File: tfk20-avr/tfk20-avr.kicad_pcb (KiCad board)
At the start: 4 copper layers, 76.2 x 115.5 mm, 123 parts, among them J1 USB_C_Receptacle_USB2.0, J2 AVR-ISP-6, SW1 Reset, U1 ATmega32U4-AU, U2 IS31FL3733-TQ, Y1 16MHz

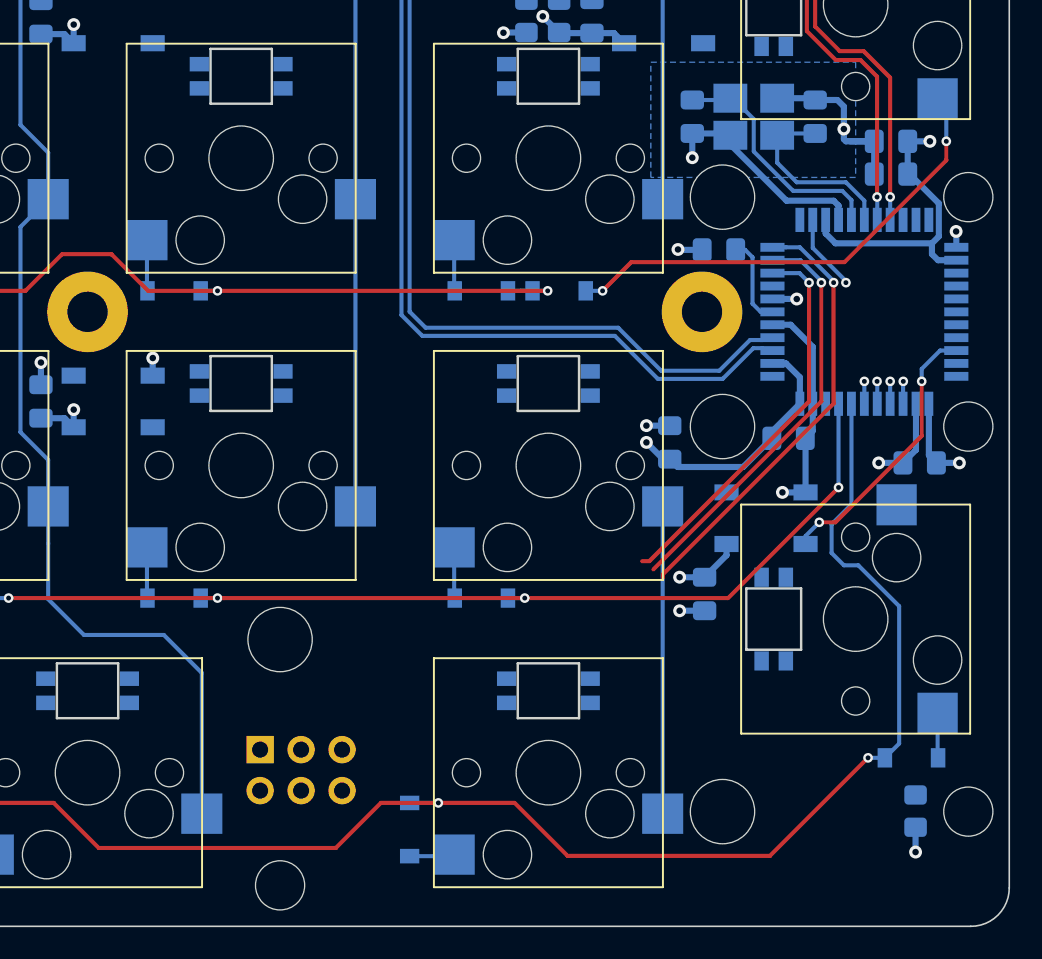
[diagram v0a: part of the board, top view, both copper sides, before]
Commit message: Continue routing
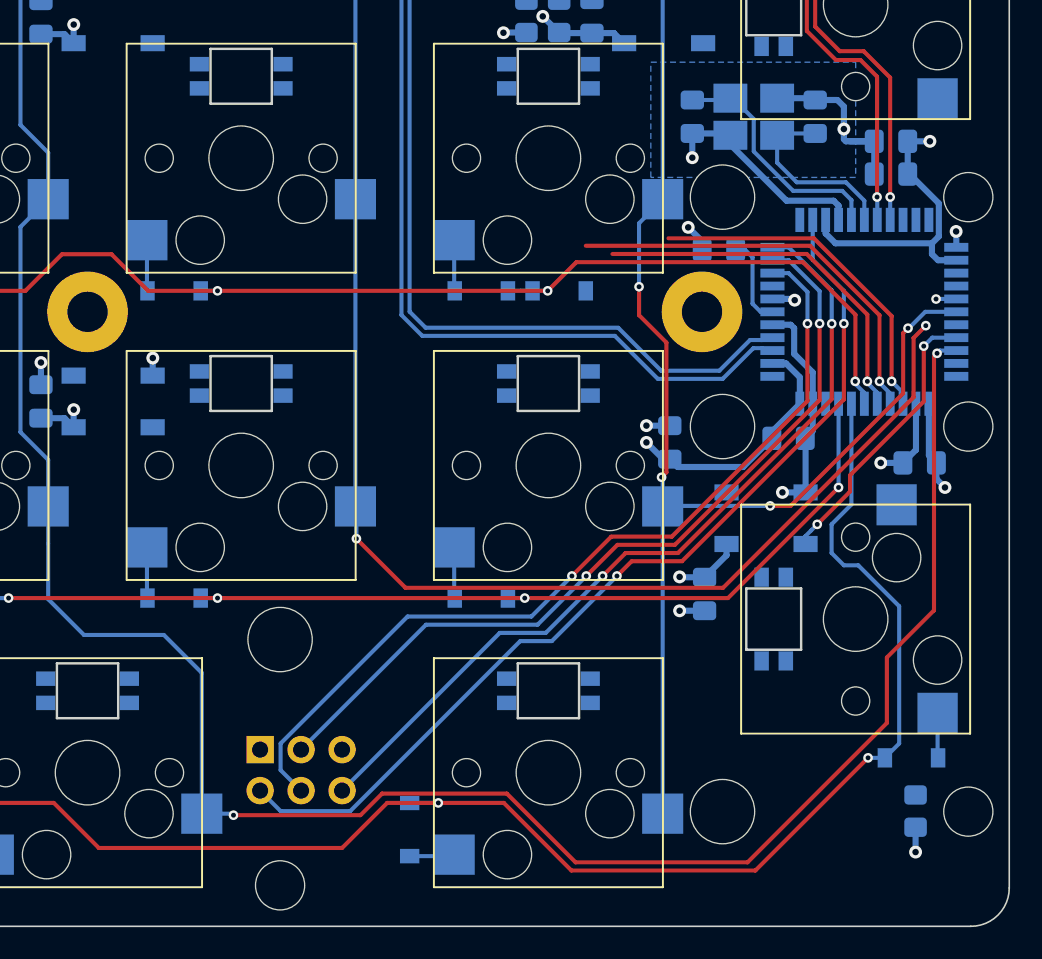
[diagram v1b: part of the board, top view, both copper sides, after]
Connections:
- U1 pad 27: /COL_2 -> /COL_3
- U1 pad 28: /COL_1 -> /COL_2
- U1 pad 29: /COL_0 -> /COL_1
- U1 pad 30: /COL_3 -> /RGB_LIGHT
- U1 pad 31: /RGB_LIGHT -> /COL_0
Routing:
- net /COL_0: track 107.8 -> 181.7 mm, vias 0 -> 2
- net /RESET: track 8.22 -> 62.7 mm, vias 2 -> 3
- net /COL_1: track 77.7 -> 125.3 mm, vias 2 -> 4
- net /COL_2: track 79.2 -> 125.1 mm, vias 0 -> 4
- net /SCK: track 24.3 -> 54.3 mm, vias 1 -> 2
- net Net-(D18-Pad2): track 29.7 -> 0.00 mm, vias 2 -> 0
- net /MOSI: track 25.8 -> 51.6 mm, vias 1 -> 2
- net /ROW_3: track 48.1 -> 73.6 mm
- net /MISO: track 27.4 -> 51.9 mm, vias 1 -> 2
- net /ROW_1: track 58.0 -> 82.4 mm
- net /ROW_2: track 43.6 -> 65.3 mm
- net /ROW_0: track 68.2 -> 88.4 mm
- net /COL_3: track 39.9 -> 41.1 mm, vias 0 -> 1
- net /ROW_5: track 91.2 -> 92.0 mm
- net /RGB_LIGHT: track 17.0 -> 17.6 mm
